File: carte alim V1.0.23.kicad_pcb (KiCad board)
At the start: 2 copper layers, 131.3 x 77.9 mm, 20 parts, among them U1 B_Plug_5mm, U10 B_Plug_5mm, U11 B_Plug_5mm, U12 B_Plug_5mm, U13 B_Plug_5mm, U2 XL4015, U3 YAAJ_DCDC_StepDown_LM2596, U4 YAAJ_DCDC_StepDown_LM2596, U5 YAAJ_DCDC_StepDown_LM2596, U6 B_Plug_5mm, U7 B_Plug_5mm, U8 B_Plug_5mm, U9 B_Plug_5mm

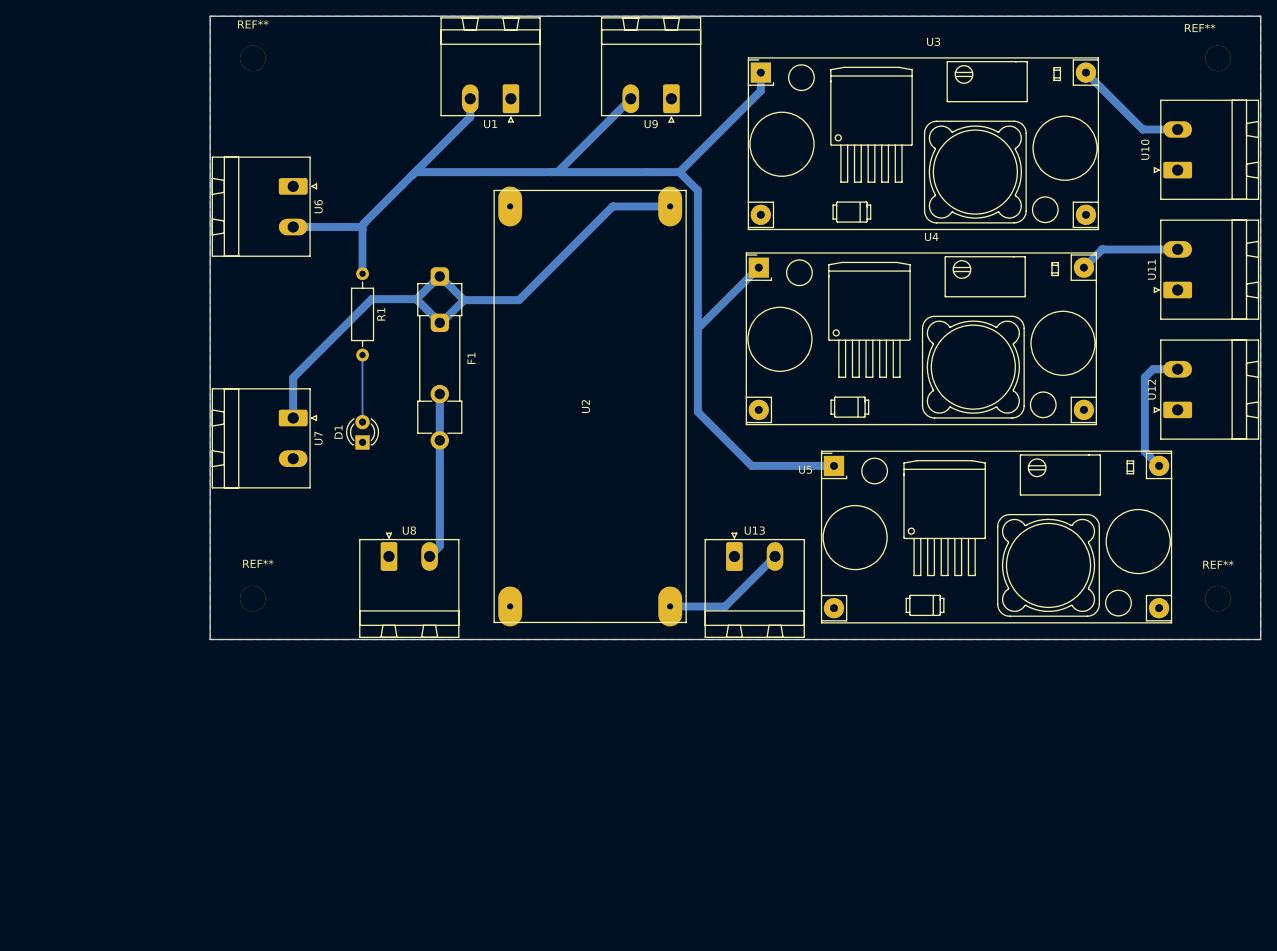
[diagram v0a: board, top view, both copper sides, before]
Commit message: new carte
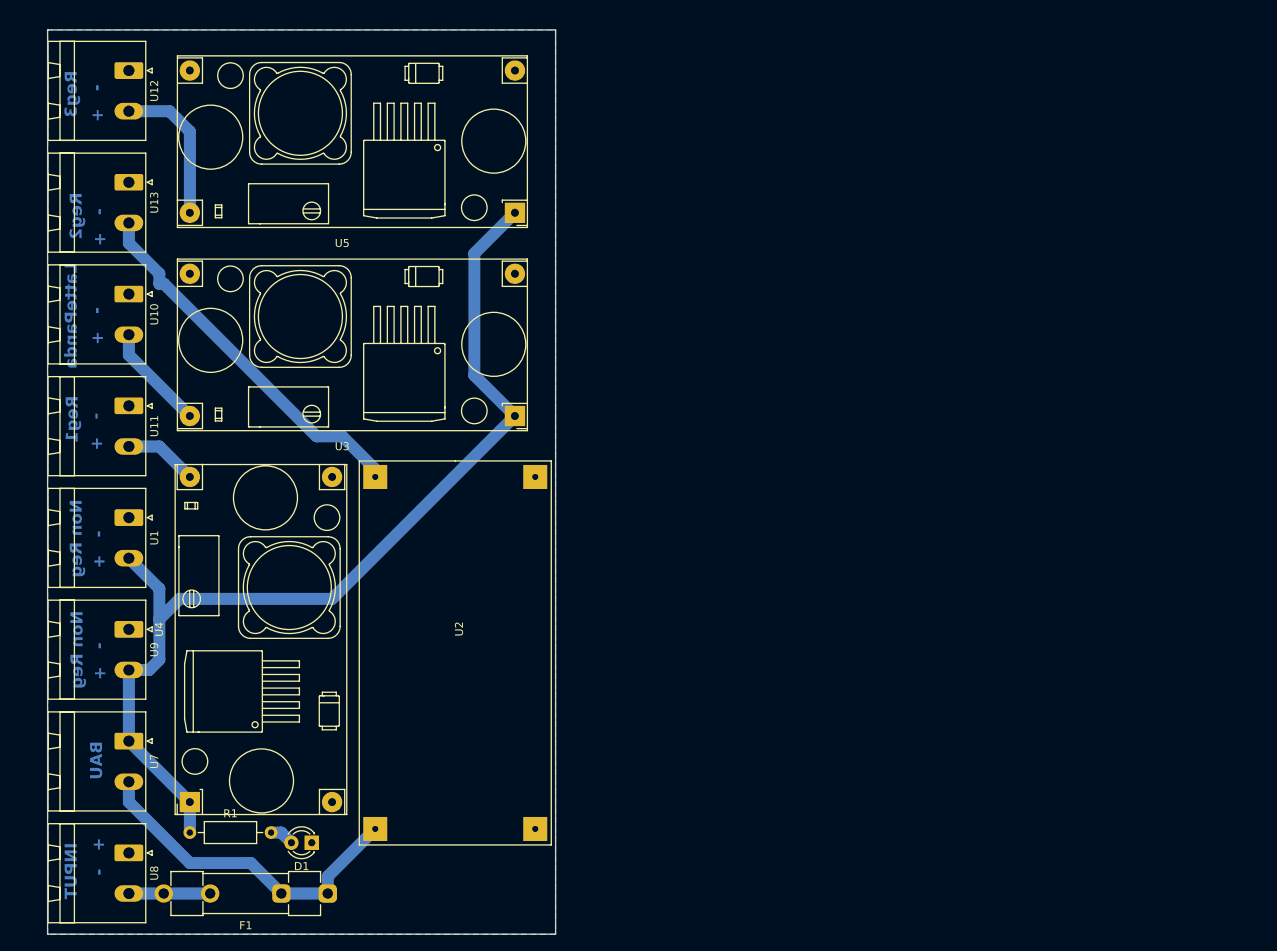
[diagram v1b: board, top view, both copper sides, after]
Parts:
- removed REF** (x4): MountingHole_3.2mm_M3, MountingHole:MountingHole_3.2mm_M3
- removed U6: B_Plug_5mm, Connector_Phoenix_MSTB:PhoenixContact_MSTBA_2,5_2-G-5,08_1x02_P5.08mm_Horizontal
- U2: footprint XL4015_converter:XL4015_Converter -> XL4015Footprint:XL4015_Converter
- moved U12 137.8 mm to (71.1, 61.0), turned to -90 degrees
- moved U10 132.0 mm to (71.1, 88.9), turned to -90 degrees
- moved U11 131.9 mm to (71.1, 102.9), turned to -90 degrees
- moved U4 97.6 mm to (78.7, 152.4), turned to 90 degrees
- moved U9 94.9 mm to (71.1, 130.8), turned to -90 degrees
- moved U13 89.0 mm to (71.1, 74.9), turned to -90 degrees
- moved F1 78.4 mm to (96.0, 163.8), turned to 180 degrees
- moved R1 73.1 mm to (78.7, 156.2), turned to 0 degrees
- moved U1 70.9 mm to (71.1, 116.8), turned to -90 degrees
- moved U3 52.8 mm to (119.4, 104.1), turned to 180 degrees
- moved U5 50.9 mm to (119.4, 78.7), turned to 180 degrees
- moved D1 50.4 mm to (94.0, 157.5), turned to 180 degrees
- moved U8 49.3 mm to (71.1, 158.8), turned to -90 degrees
- moved U7 45.3 mm to (71.1, 144.8)
- moved U2 32.5 mm to (111.9, 130.8), turned to 90 degrees
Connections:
- U7 pad 1: Net-(U2-IN+) -> Net-(U3-Vin)
- U7 pad 2: GND -> Net-(U2-IN+)
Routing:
- net Net-(U3-Vin): track 161.2 -> 126.7 mm
- net Net-(U2-OUT+): track 15.7 -> 46.7 mm
- net Net-(U2-IN+): track 71.9 -> 42.7 mm
- net 14.4_VBattery: track 20.8 -> 10.2 mm
- net Net-(D1-A): track 8.38 -> 3.07 mm
- net Net-(U4-Vout): track 12.7 -> 9.20 mm
- net Net-(U5-Vout): track 16.3 -> 18.8 mm
- net Regulated_motor: track 14.4 -> 13.3 mm
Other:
- board size 131.3 x 77.9 mm -> 63.5 x 113 mm
- board text added: "+ -"
- board text added: "BAU"
- board text added: "INPUT"
- board text added: "LattePanda"
- board text added: "Non Reg"
- board text added: "Reg1"
- board text added: "Reg2"
- board text added: "Reg3"

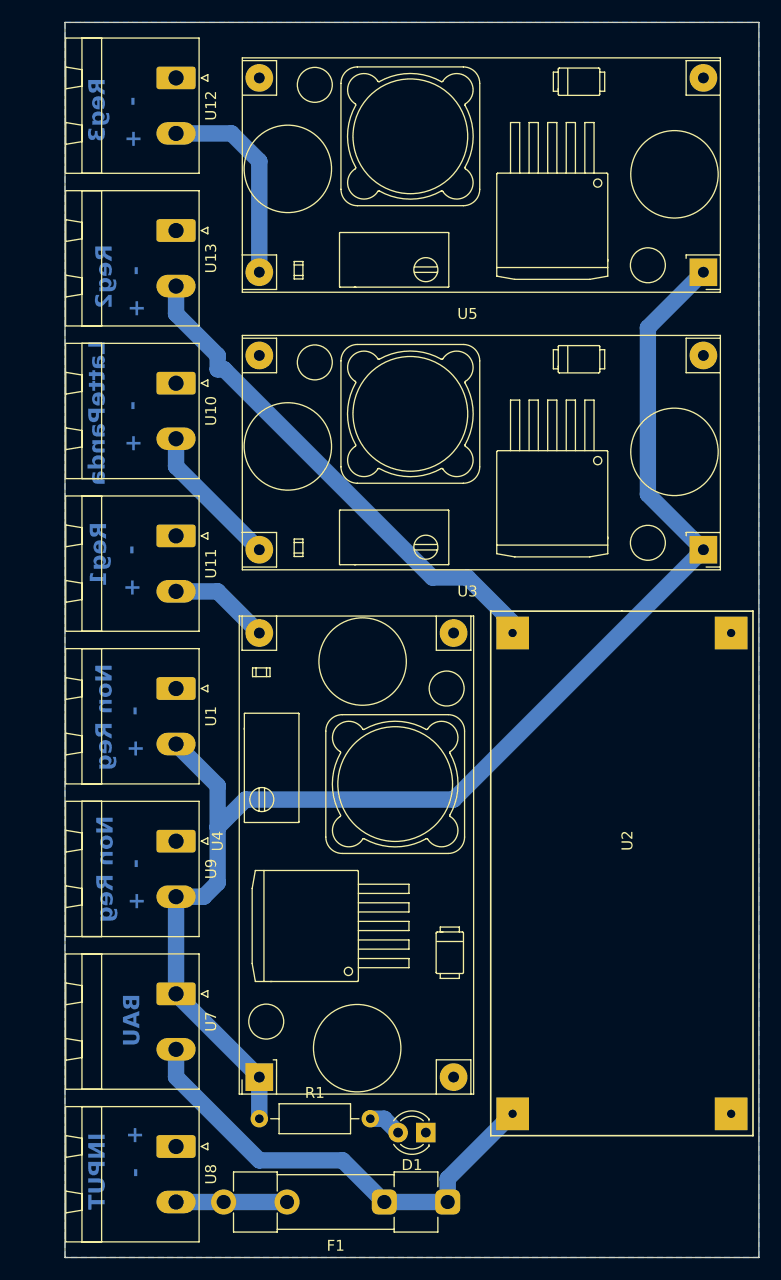
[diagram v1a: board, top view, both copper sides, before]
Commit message: carte final V3
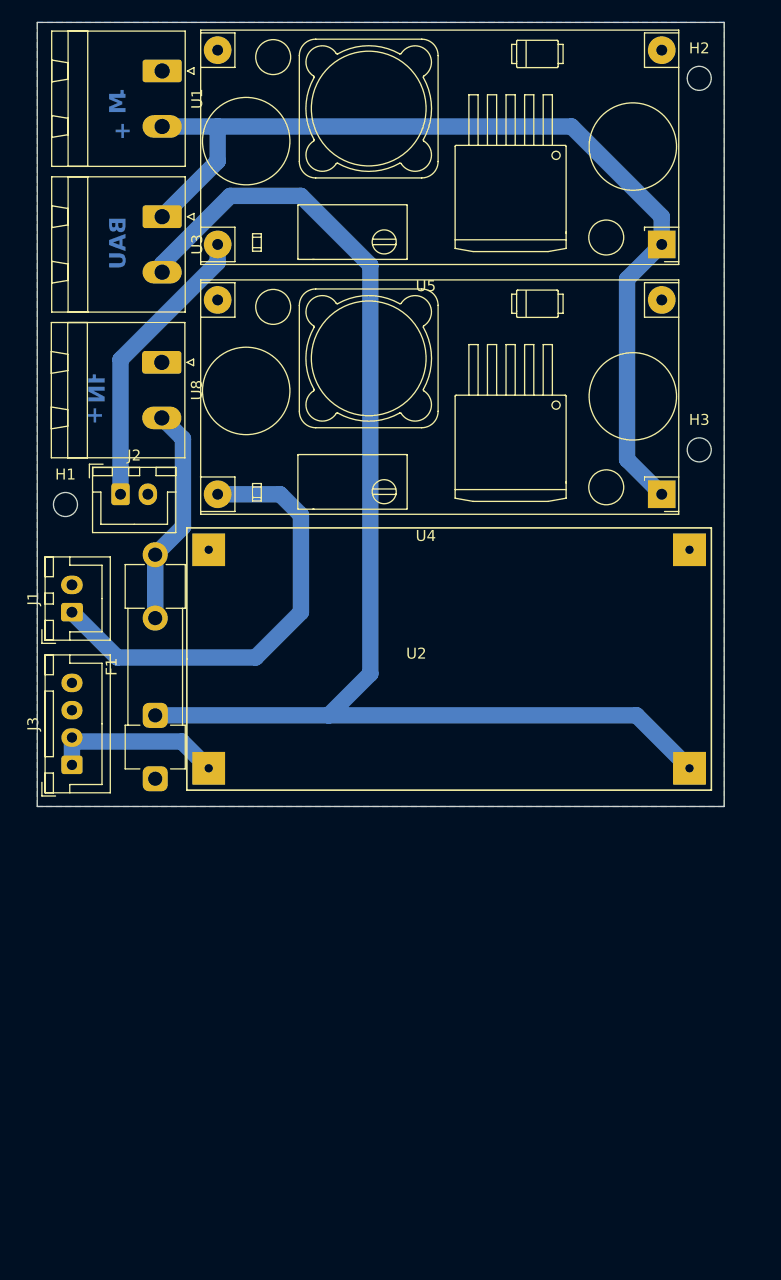
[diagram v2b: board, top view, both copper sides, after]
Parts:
- removed D1: LED, LED_THT:LED_D3.0mm
- removed R1: R, Resistor_THT:R_Axial_DIN0207_L6.3mm_D2.5mm_P10.16mm_Horizontal
- removed U10, U11, U12, U13, U7, U9: B_Plug_5mm, Connector_Phoenix_MSTB:PhoenixContact_MSTBA_2,5_2-G-5,08_1x02_P5.08mm_Horizontal
- added H1: MountingHole, MountingHole:MountingHole_2.2mm_M2_ISO7380, F.Cu at (61.0, 100.0)
- added H2: MountingHole, MountingHole:MountingHole_2.2mm_M2_ISO7380, F.Cu at (119.0, 61.0)
- added H3: MountingHole, MountingHole:MountingHole_2.2mm_M2_ISO7380, F.Cu at (119.0, 95.0)
- added J1: Conn_01x02, Connector_JST:JST_XH_B2B-XH-A_1x02_P2.50mm_Vertical, F.Cu at (61.6, 109.9)
- added J2: Conn_01x02, Connector_JST:JST_XH_B2B-XH-A_1x02_P2.50mm_Vertical, F.Cu at (66.0, 99.1)
- added J3: Conn_01x04, Connector_JST:JST_XH_B4B-XH-A_1x04_P2.50mm_Vertical, F.Cu at (61.6, 123.8)
- U3: value YAAJ_DCDC_StepDown_LM2596 -> B_Plug_5mm; footprint Footprints:YAAJ_DCDC_StepDown_LM2596 -> Connector_Phoenix_MSTB:PhoenixContact_MSTBA_2,5_2-G-5,08_1x02_P5.08mm_Horizontal
- moved U8 71.8 mm to (69.8, 87.0)
- moved U4 64.8 mm to (115.6, 99.1), turned to 180 degrees
- moved U3 58.2 mm to (69.8, 73.7), turned to -90 degrees
- moved U1 56.5 mm to (69.8, 60.3)
- moved F1 47.1 mm to (69.2, 125.1), turned to 90 degrees
- moved U2 25.1 mm to (93.1, 114.1), turned to 180 degrees
- moved U5 4.58 mm to (115.6, 76.2)
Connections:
- U3 pad 2: GND -> Net-(U2-IN+)
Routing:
- net Net-(U2-IN+): track 42.7 -> 118.7 mm
- net Net-(U4-Vin): track 126.7 -> 87.5 mm
- net Net-(J1-Pin_1): track 9.20 -> 41.7 mm
- net Net-(J3-Pin_1): track 46.7 -> 16.2 mm
- net Regulated_motor: track 13.3 -> 0.00 mm
- net 14.4_VBattery: track 10.2 -> 20.2 mm
- net Net-(J2-Pin_1): track 18.8 -> 26.5 mm
- net Net-(D1-A): track 3.07 -> 0.00 mm
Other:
- board size 63.5 x 113 mm -> 62.9 x 71.8 mm
- board text added: "IN"
- board text added: "M"
- board text removed: "INPUT"
- board text removed: "LattePanda"
- board text removed: "Non Reg"
- board text removed: "Reg1"
- board text removed: "Reg2"
- board text removed: "Reg3"
